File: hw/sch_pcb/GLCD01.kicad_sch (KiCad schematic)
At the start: 8 parts, among them J1 Umin ... Umax, M1 HOLE M3, M2 HOLE M3, M3 HOLE, M4 HOLE

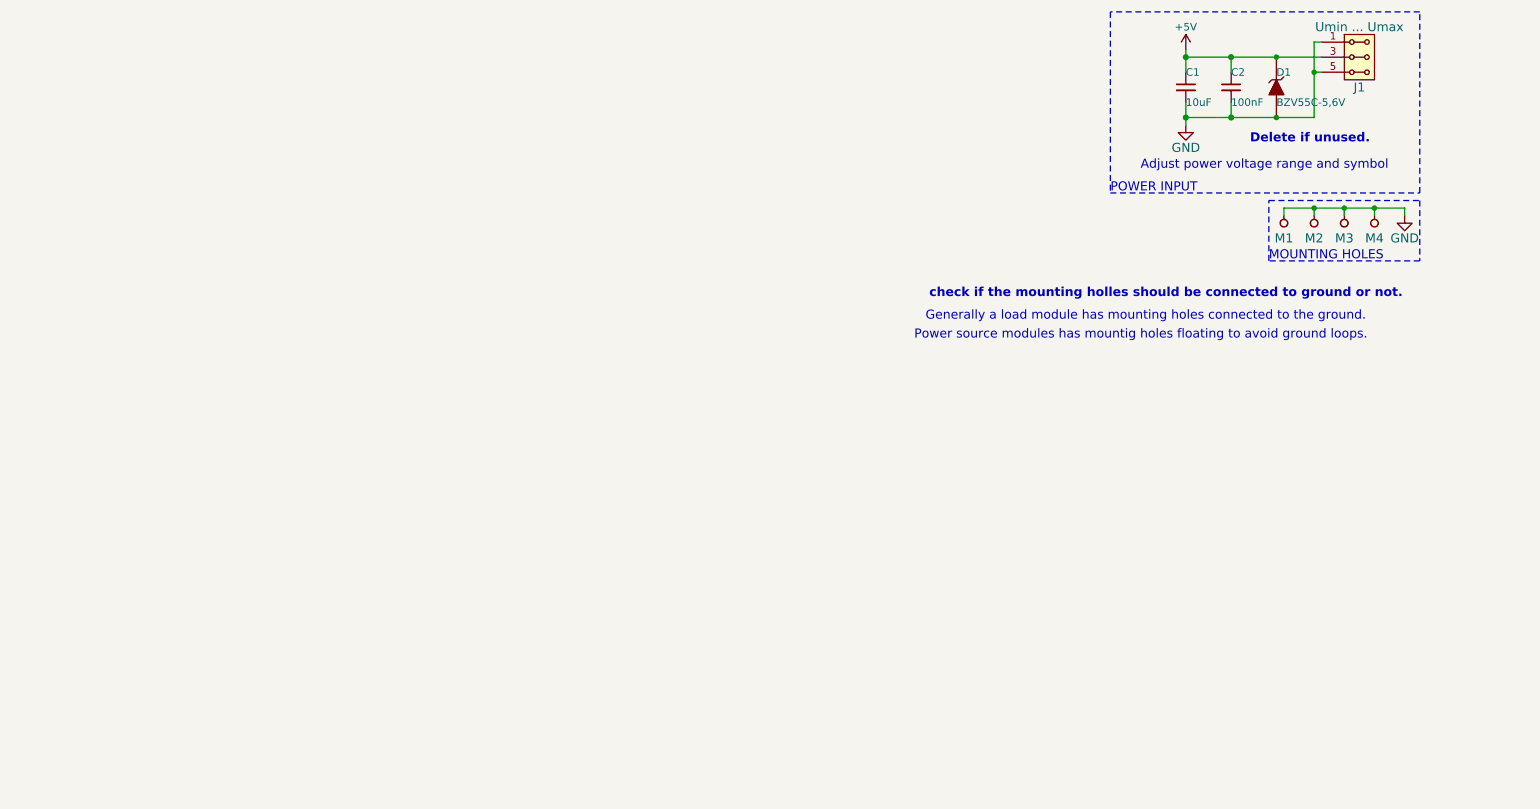
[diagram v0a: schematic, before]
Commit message: v1 with mic1557
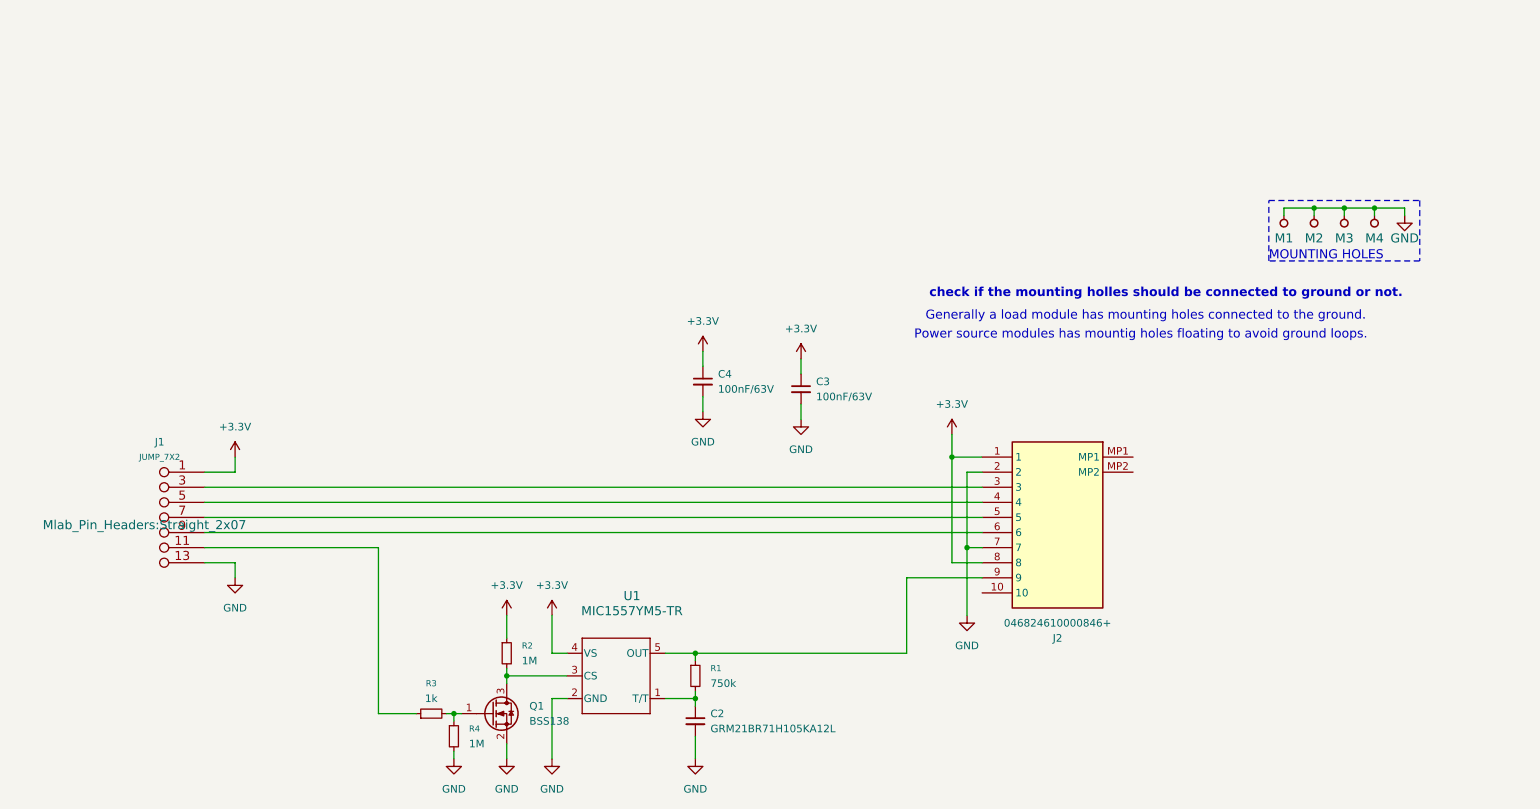
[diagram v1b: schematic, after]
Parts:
- removed C1: 10uF, Capacitor_SMD:C_0805_2012Metric, symbol ISM02A-rescue:C_Small-Device-ISM02A-rescue
- removed C2: 100nF, Capacitor_SMD:C_0805_2012Metric, symbol ISM02A-rescue:C_Small-Device-ISM02A-rescue
- removed D1: BZV55C-5,6V, Diode_SMD:D_SMA, symbol ISM02A-rescue:D_ZENER-MLAB_D
- removed J1: Umin ... Umax, Mlab_Pin_Headers:Straight_2x03, symbol header:HEADER_2x03_PARALLEL
- added C2: GRM21BR71H105KA12L, Capacitor_SMD:C_0603_1608Metric, symbol Device:C_Small
- added C3, C4: 100nF/63V, Capacitor_SMD:C_0603_1608Metric, symbol Device:C_Small
- added J1: JUMP_7X2, Mlab_Pin_Headers:Straight_2x07, symbol MLAB_Jumpers:JUMP_7X2
- added J2: 046824610000846+, 046824610000846, symbol FPC_10:046824610000846+
- added Q1: BSS138, Package_TO_SOT_SMD:SOT-23, symbol Transistor_FET:BSS138
- added R1: 750k, Resistor_SMD:R_0603_1608Metric, symbol Device:R_Small
- added R2, R4: 1M, Resistor_SMD:R_0603_1608Metric, symbol Device:R_Small
- added R3: 1k, Resistor_SMD:R_0603_1608Metric, symbol Device:R_Small
- added U1: MIC1557YM5-TR, Package_TO_SOT_SMD:SOT-23-5, symbol MIC1557:MIC1557YM5-TR
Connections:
- net GND: now also C2.2, C3.2, C4.2, J1.13 (14), J1.14, J2.2, J2.7, Q1.2 (S), R4.2, U1.2 (GND)
- new net: Q1.3 (D), R2.2, U1.3 (CS)
- new net: J1.10, J1.9 (10), J2.6
- new net: J1.11 (12), J1.12, R3.1
- new net: J1.3 (4), J1.4, J2.3
- new net: J1.5 (6), J1.6, J2.4
- new net: J1.7 (8), J1.8, J2.5
- new net: Q1.1 (G), R3.2, R4.1
- new net: J2.9, R1.1, U1.5 (OUT)
- new net: C2.1, R1.2, U1.1 (T/T)
- new net +3.3V: C3.1, C4.1, J1.1 (2), J1.2, J2.1, J2.8, R2.1, U1.4 (VS)
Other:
- note removed: "Adjust power voltage range and symbol"
- note removed: "Delete if unused."
- note removed: "POWER INPUT"
